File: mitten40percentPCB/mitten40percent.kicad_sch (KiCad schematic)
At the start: 10 parts, among them SW1 SW_Push, U1 STM32F072CBT6

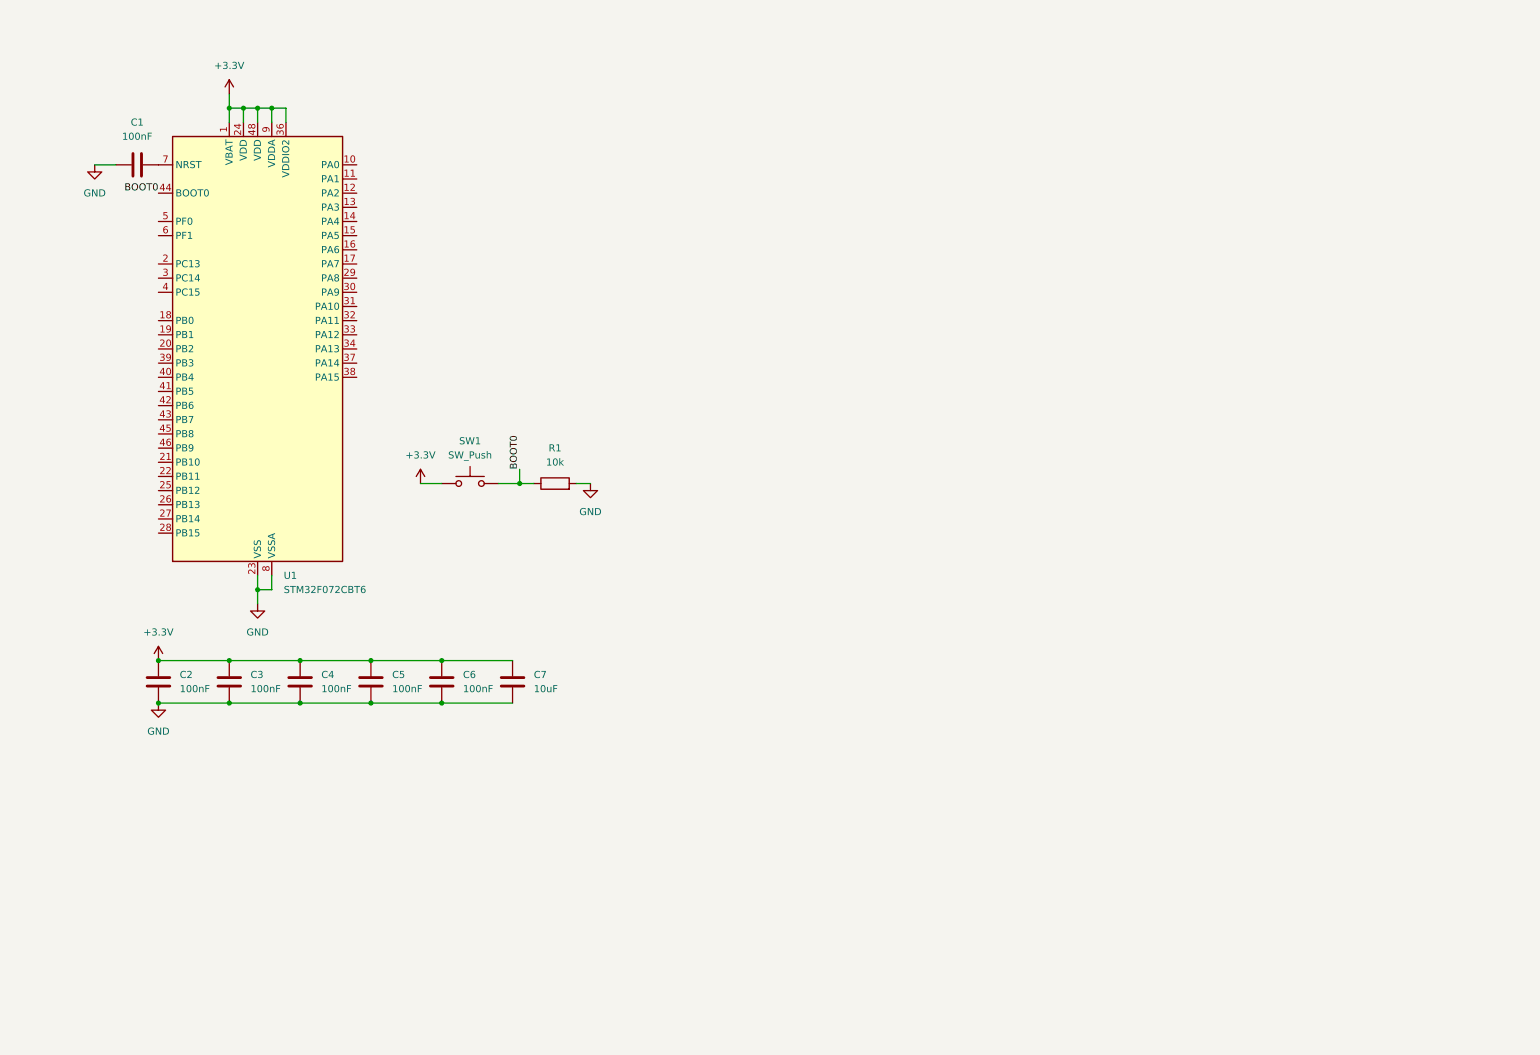
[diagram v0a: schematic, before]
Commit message: stm32 wiring finally finished!!!! (theres a non-zero percent chance it will burn my house down)
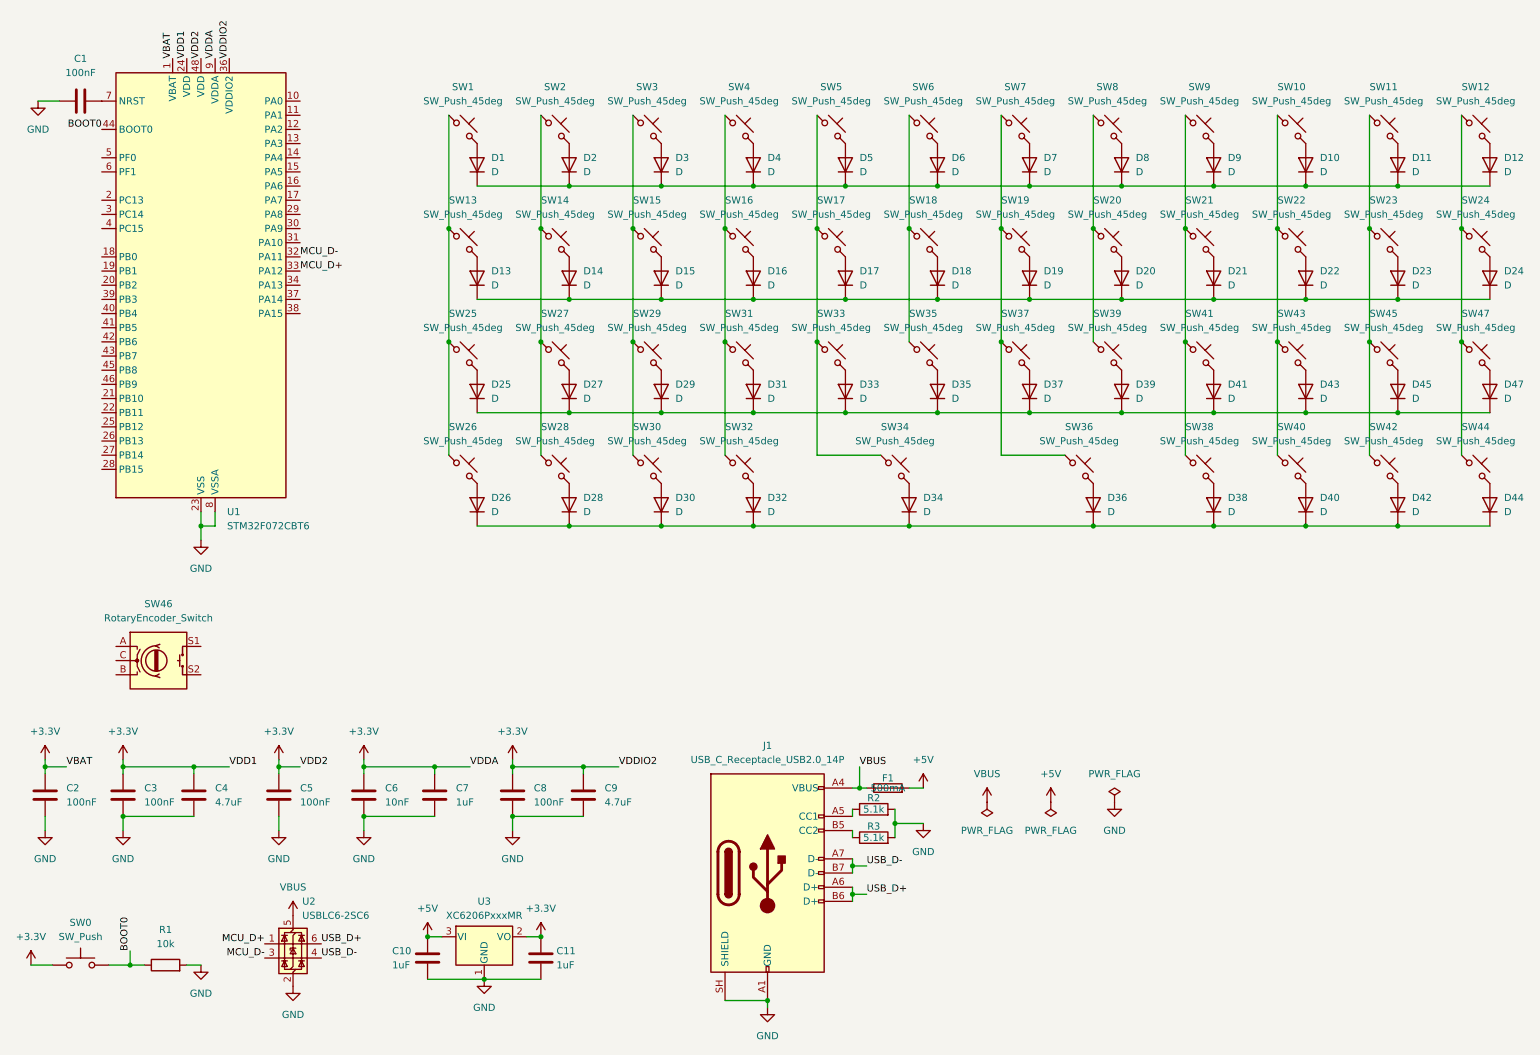
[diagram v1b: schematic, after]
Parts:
- added C10, C11: 1uF, symbol Device:C
- added C8: 100nF, symbol Device:C
- added C9: 4.7uF, symbol Device:C
- added D1, D10, D11, D12, D13, D14, D15, D16, D17, D18, D19, D2, D20, D21, D22, D23, D24, D25, D26, D27, D28, D29, D3, D30, D31, D32, D33, D34, D35, D36, D37, D38, D39, D4, D40, D41, D42, D43, D44, D45, D47, D5, D6, D7, D8, D9: D, symbol Device:D
- added F1: 500mA, symbol Device:Fuse
- added J1: USB_C_Receptacle_USB2.0_14P, symbol Connector:USB_C_Receptacle_USB2.0_14P
- added R2, R3: 5.1k, symbol Device:R
- added SW1, SW10, SW11, SW12, SW13, SW14, SW15, SW16, SW17, SW18, SW19, SW2, SW20, SW21, SW22, SW23, SW24, SW25, SW26, SW27, SW28, SW29, SW3, SW30, SW31, SW32, SW33, SW34, SW35, SW36, SW37, SW38, SW39, SW4, SW40, SW41, SW42, SW43, SW44, SW45, SW47, SW5, SW6, SW7, SW8, SW9: SW_Push_45deg, symbol Switch:SW_Push_45deg
- added SW46: RotaryEncoder_Switch, symbol Device:RotaryEncoder_Switch
- added U2: USBLC6-2SC6, Package_TO_SOT_SMD:SOT-23-6, symbol Power_Protection:USBLC6-2SC6
- added U3: XC6206PxxxMR, Package_TO_SOT_SMD:SOT-23-3, symbol Regulator_Linear:XC6206PxxxMR
- C4: value 100nF -> 4.7uF
- C6: value 100nF -> 10nF
- C7: value 10uF -> 1uF
- renumbered SW1 to SW0
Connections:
- net +3.3V: now also C11.1, C8.1, C9.1, U3.2 (VO)
- net GND: now also C10.2, C11.2, C8.2, C9.2, J1.A1 (GND), J1.A12 (GND), J1.B1 (GND), J1.B12 (GND), J1.SH (SHIELD), R2.2, R3.2, U2.2 (GND), U3.1 (GND)
- net MCU_D-: now reaches U1.32 (PA11)
- net MCU_D-: now also U2.3 (I/O2)
- net MCU_D+: now reaches U1.33 (PA12)
- net MCU_D+: now also U2.1 (I/O1)
- new net: SW19.1, SW36.1, SW37.1, SW7.1
- new net: D19.2 (A), SW19.2
- new net: SW1.1, SW13.1, SW25.1, SW26.1
- new net: D13.2 (A), SW13.2
- new net: D1.1 (K), D10.1 (K), D11.1 (K), D12.1 (K), D2.1 (K), D3.1 (K), D4.1 (K), D5.1 (K), D6.1 (K), D7.1 (K), D8.1 (K), D9.1 (K)
- new net: D5.2 (A), SW5.2
- new net: D26.1 (K), D28.1 (K), D30.1 (K), D32.1 (K), D34.1 (K), D36.1 (K), D38.1 (K), D40.1 (K), D42.1 (K), D44.1 (K)
- new net: D44.2 (A), SW44.2
- new net: SW16.1, SW31.1, SW32.1, SW4.1
- new net: D4.2 (A), SW4.2
- new net: D30.2 (A), SW30.2
- new net: D1.2 (A), SW1.2
- new net: SW20.1, SW39.1, SW8.1
- new net: D20.2 (A), SW20.2
- new net: SW10.1, SW22.1, SW40.1, SW43.1
- new net: D22.2 (A), SW22.2
- new net: D13.1 (K), D14.1 (K), D15.1 (K), D16.1 (K), D17.1 (K), D18.1 (K), D19.1 (K), D20.1 (K), D21.1 (K), D22.1 (K), D23.1 (K), D24.1 (K)
- new net: D14.2 (A), SW14.2
- new net: D24.2 (A), SW24.2
- new net: D10.2 (A), SW10.2
- new net: SW18.1, SW35.1, SW6.1
- new net: D18.2 (A), SW18.2
- new net: D28.2 (A), SW28.2
- new net: D25.1 (K), D27.1 (K), D29.1 (K), D31.1 (K), D33.1 (K), D35.1 (K), D37.1 (K), D39.1 (K), D41.1 (K), D43.1 (K), D45.1 (K), D47.1 (K)
- new net: D25.2 (A), SW25.2
- new net: D40.2 (A), SW40.2
- new net: SW15.1, SW29.1, SW3.1, SW30.1
- new net: D15.2 (A), SW15.2
- new net: D3.2 (A), SW3.2
- new net: D16.2 (A), SW16.2
- new net: SW14.1, SW2.1, SW27.1, SW28.1
- new net: D7.2 (A), SW7.2
- new net: D35.2 (A), SW35.2
- new net: SW21.1, SW38.1, SW41.1, SW9.1
- new net: D38.2 (A), SW38.2
- new net: D11.2 (A), SW11.2
- new net: D43.2 (A), SW43.2
- new net: SW12.1, SW24.1, SW44.1, SW47.1
- new net: D12.2 (A), SW12.2
- new net: D17.2 (A), SW17.2
- new net: D47.2 (A), SW47.2
- new net: D41.2 (A), SW41.2
- new net: D36.2 (A), SW36.2
- new net: D45.2 (A), SW45.2
- new net: SW11.1, SW23.1, SW42.1, SW45.1
- new net: D6.2 (A), SW6.2
- new net: D23.2 (A), SW23.2
- new net: D33.2 (A), SW33.2
- new net: SW17.1, SW33.1, SW34.1, SW5.1
- new net: D2.2 (A), SW2.2
- new net: D39.2 (A), SW39.2
- new net: D31.2 (A), SW31.2
- new net: D29.2 (A), SW29.2
- new net: D27.2 (A), SW27.2
- new net: D34.2 (A), SW34.2
- new net: D37.2 (A), SW37.2
- new net: D8.2 (A), SW8.2
- new net: D32.2 (A), SW32.2
- new net: J1.A5 (CC1), R2.1
- new net: J1.B5 (CC2), R3.1
- new net: D26.2 (A), SW26.2
- new net: D9.2 (A), SW9.2
- new net: D42.2 (A), SW42.2
- new net: D21.2 (A), SW21.2
- new net +5V: C10.1, F1.2, U3.3 (VI)
- new net USB_D+: J1.A6 (D+), J1.B6 (D+), U2.6 (I/O1)
- new net USB_D-: J1.A7 (D-), J1.B7 (D-), U2.4 (I/O2)
- new net VBUS: F1.1, J1.A4 (VBUS), J1.A9 (VBUS), J1.B4 (VBUS), J1.B9 (VBUS), U2.5 (VBUS)
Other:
- moved on the sheet: C1, R1, SW0, U1
